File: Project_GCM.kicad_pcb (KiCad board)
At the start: 4 copper layers, 203 x 116 mm, 127 parts, among them J1 Molex_1053102116, J10 MM1_addressExtension, J11 MM1_receptacle_5530843-2, J12 DEBUG_BUSES, J13 MM1_addressExtension, J2 PP1_receptacle_TE_5-5530843-4, J3 PP1_receptacle_TE_5-5530843-4, J4 PP1_receptacle_TE_5-5530843-4, J5 PP1_receptacle_TE_5-5530843-4, J6 TE_Eurocard_96pole, J7 3-641124-6, J8 MM1_receptacle_5530843-2, J9 Conn_01x02, U1 LM810, U10 74LVC1G74, U11 74AHC1G04, U12 74AHC244, U13 CD74AC161M, U14 CD74AC161M, U15 74AHCT1G04, U16 CD74AC161M, U17 CD74AC161M, U18 74AHC1G04, U19 CD74AC161M, U2 LTC6994xS6-1, U20 CD74AC161M, U21 74AHCT244, U22 74CBTLV16212, U23 74CBTLV16212, U24 74CBTLV16212, U25 74AHC1G32, U26 SN74LV393A, U27 SN74LV393A, U28 CD74AC151, U29 CD74AC151, U3 74AHC1G32, U30 74AHC1G32, U31 CD74AC151, U32 74AHC273, U33 SN74LV393A, U34 SN74LV393A, U35 CD74AC151, U36 CD74AC151, U37 CD74AC151, U4 74AHC273, U40 74AHC273, U41 74AHC1G04, U42 74AHC273, U43 74AHC273, U44 74AHC273, U5 74AHC1G04, U6 CD74AC238, U7 74AHC138, U8 74AHC244, U9 74AHC244, X1 ECS-2200BX-500

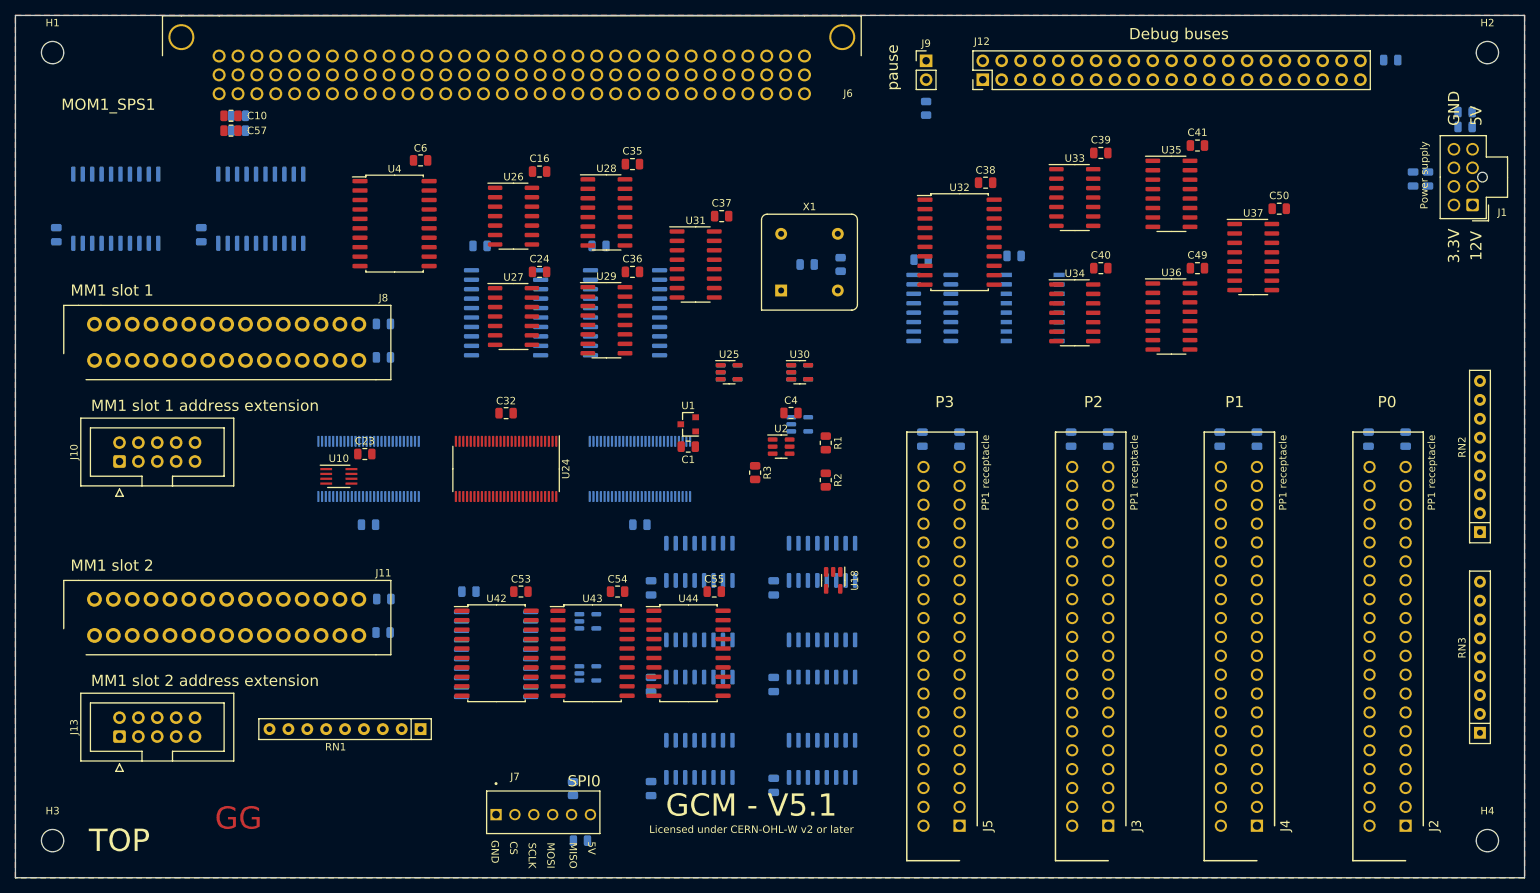
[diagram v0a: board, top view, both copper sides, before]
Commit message: First step, import ses
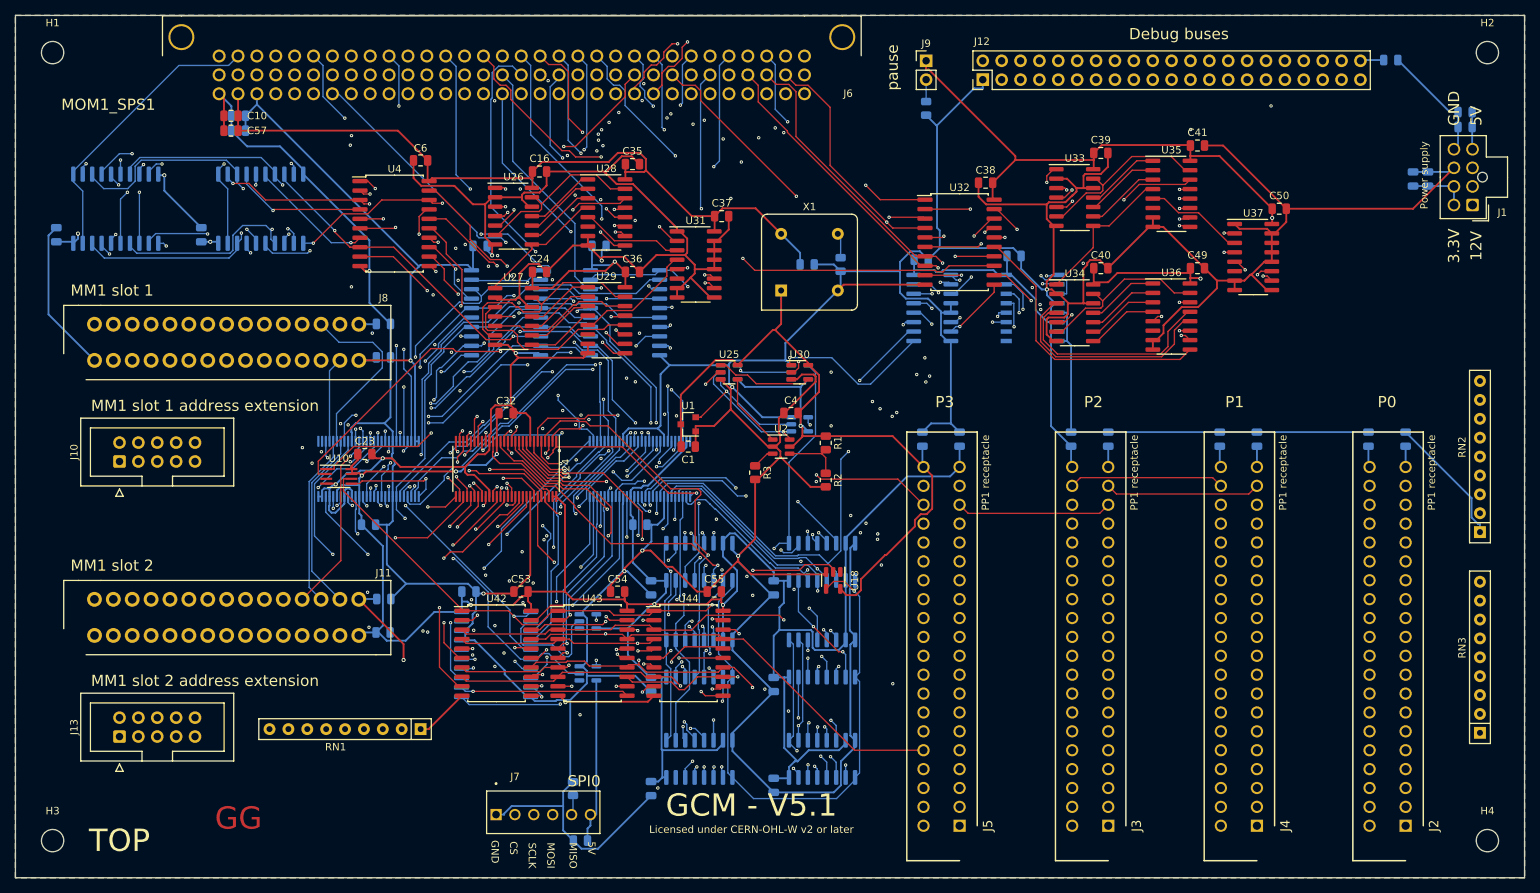
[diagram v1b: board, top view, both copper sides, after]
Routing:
- net GND: track 0.00 -> 1410.1 mm, vias 0 -> 14
- net +5V: track 0.00 -> 755.6 mm, vias 0 -> 7
- net +3V3: track 0.00 -> 540.7 mm, vias 0 -> 7
- net /ClockGenerator/BWRITE1_0: track 0.00 -> 328.9 mm, vias 0 -> 8
- net /ClockGenerator/BWRITE1_4: track 0.00 -> 322.5 mm, vias 0 -> 5
- net /ClockGenerator/BWRITE1_5: track 0.00 -> 311.1 mm, vias 0 -> 6
- net /ClockGenerator/BWRITE1_1: track 0.00 -> 298.9 mm, vias 0 -> 6
- net /ClockGenerator/BWRITE1_2: track 0.00 -> 297.6 mm, vias 0 -> 5
- net /Connector/BWRITE2_0: track 0.00 -> 291.3 mm, vias 0 -> 3
- net /Connector/BWRITE2_2: track 0.00 -> 288.6 mm, vias 0 -> 4
- net /ClockGenerator/BWRITE1_3: track 0.00 -> 288.3 mm, vias 0 -> 5
- net /Connector/BWRITE2_4: track 0.00 -> 284.5 mm, vias 0 -> 5
- net /Connector/BWRITE2_6: track 0.00 -> 282.0 mm, vias 0 -> 2
- net /Connector/BWRITE2_1: track 0.00 -> 278.8 mm, vias 0 -> 3
- net /Connector/BWRITE2_3: track 0.00 -> 276.9 mm, vias 0 -> 4
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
